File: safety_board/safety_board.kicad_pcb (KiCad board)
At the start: 2 copper layers, 201.2 x 121.8 mm, 74 parts, among them J1 430450200, J12 XT60-M, J13 XT60-M, J15 22035035, J18 XT60-M, J2 430450200, J3 22035035, J4 22035035, J5 22035035, J6 22035035, J7 XT60-M, J8 22035035, J9 430450200, U1 LDL1117S50R, U14 J115F11AH12VDCS61.5U, U15 J115F11AH12VDCS61.5U, U19 J115F11AH12VDCS61.5U, U2 IRLML6344TRPBF, U4 IRLML6344TRPBF, U5 J115F11AH12VDCS61.5U, U6 J115F11AH12VDCS61.5U, U7 SN74HCS21QPWRQ1

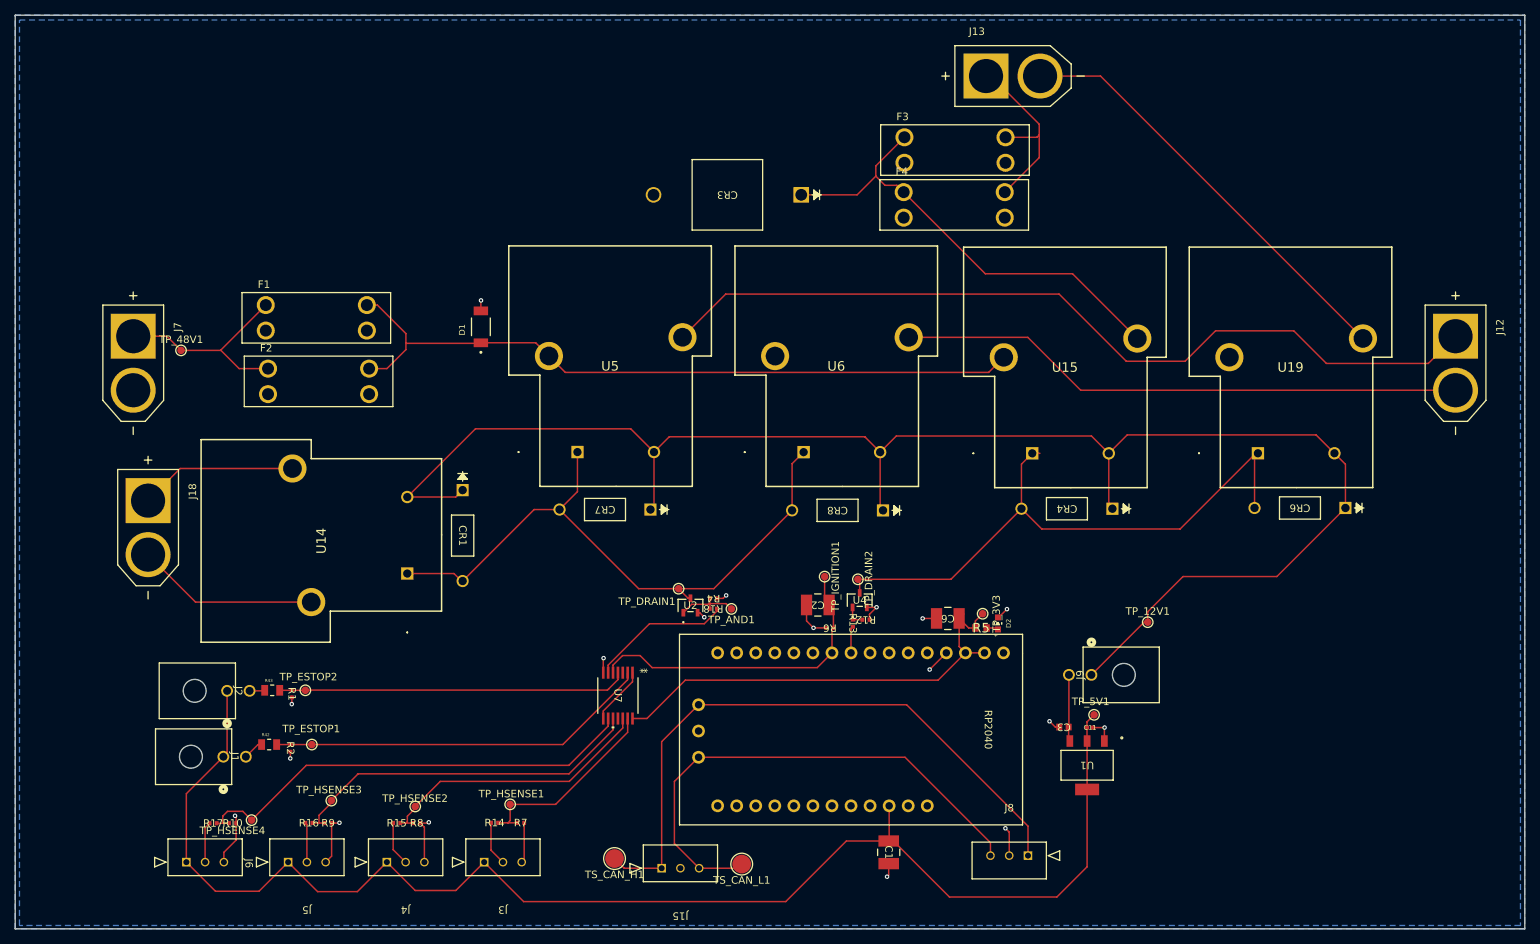
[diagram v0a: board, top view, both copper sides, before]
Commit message: maybe possibly final
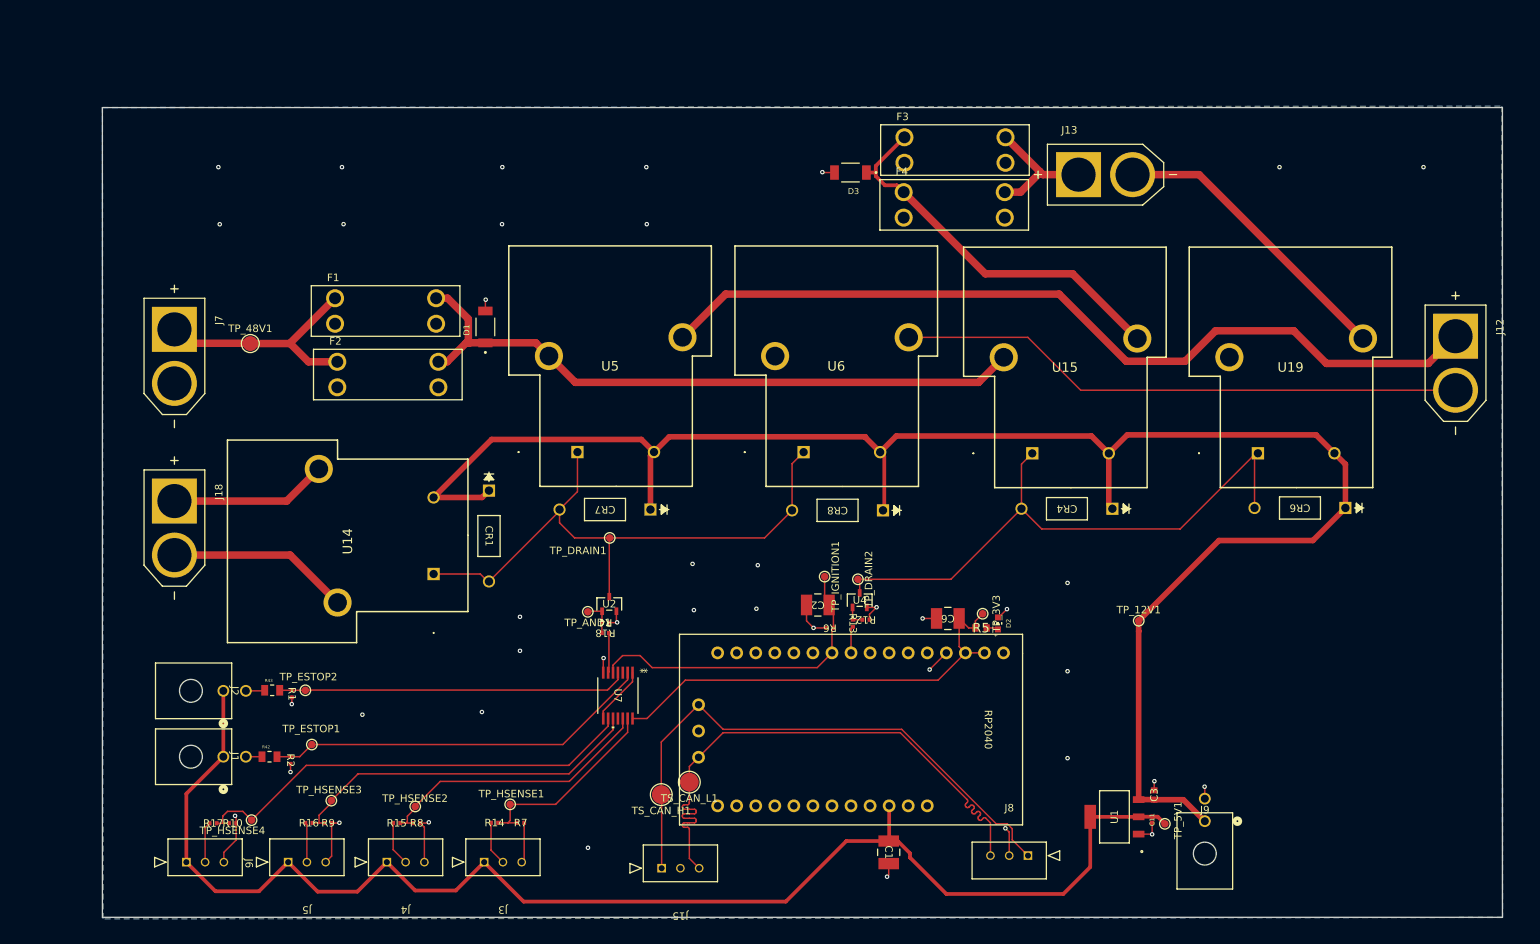
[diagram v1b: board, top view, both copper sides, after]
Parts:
- removed CR3: 5KP48A, SMV_Passives:DIODE_P600_VIS
- added D3: SMA4S56AH, SMV_Passives:SODFL4725X110N, F.Cu at (153.2, 55.9)
- TP_48V1: footprint TestPoint:TestPoint_Pad_D1.0mm -> TestPoint:TestPoint_Pad_D2.0mm
- moved J9 24.7 mm to (200.4, 142.3), turned to 0 degrees
- moved TP_AND1 19.1 mm to (118.2, 114.4)
- moved J13 18.0 mm to (187.2, 56.2)
- moved TP_5V1 17.3 mm to (195.1, 142.7), turned to 90 degrees
- moved C3 15.1 mm to (193.6, 138.9), turned to 90 degrees
- moved C11 14.8 mm to (193.4, 142.1), turned to -90 degrees
- moved R18 14.7 mm to (120.5, 117.3)
- moved R4 14.7 mm to (120.5, 115.9)
- moved TS_CAN_L1 13.0 mm to (131.7, 137.1)
- moved TP_DRAIN1 11.4 mm to (121.1, 104.6)
- moved U2 10.8 mm to (121.0, 113.4)
- moved TS_CAN_H1 10.6 mm to (127.9, 138.8)
- moved F1 9.27 mm to (91.2, 74.3)
- moved F2 9.27 mm to (91.5, 82.8)
- moved TP_48V1 9.27 mm to (73.2, 78.7)
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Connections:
- net /CAN_H renamed /CAN_P
- net /CAN_L renamed /CAN_N
- C3 pad 1: Net-(U1-VIN) -> +12V
- J9 pad 2: Net-(U1-VIN) -> GND
- U1 pad 3: Net-(U1-VIN) -> +12V
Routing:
- net +12V: track 217.1 -> 236.4 mm
- net Net-(J13-NEG): track 57.5 -> 39.7 mm
- net Net-(U7-1Y): track 18.8 -> 5.33 mm
- net Net-(U15-NO): track 61.5 -> 51.9 mm
- net Net-(U1-VIN): track 8.90 -> 0.00 mm
- net Net-(U15-COM): track 97.0 -> 88.7 mm
- net /CAN_P: track 85.2 -> 77.0 mm
- net /CAN_N: track 68.7 -> 76.7 mm
- net Net-(J13-POS): track 25.4 -> 17.7 mm
- net Net-(J7-POS): track 28.3 -> 32.0 mm
- net Net-(U2-G): track 8.58 -> 4.86 mm
- net +5V: track 190.4 -> 186.9 mm
- net GND: track 60.6 -> 63.9 mm, vias 18 -> 41
- net /DRAIN: track 83.5 -> 81.3 mm
- net /DRAIN2: track 80.9 -> 79.9 mm
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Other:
- board size 201.2 x 121.8 mm -> 186.6 x 107.9 mm
